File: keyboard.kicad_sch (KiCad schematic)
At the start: 101 parts, among them SW1 SW_PUSH, SW10 SW_PUSH, SW11 SW_PUSH, SW12 SW_PUSH, SW13 SW_PUSH, SW14 SW_PUSH, SW15 SW_PUSH, SW16 SW_PUSH, SW17 SW_PUSH, SW18 SW_PUSH, SW19 SW_PUSH, SW2 SW_PUSH, SW20 SW_PUSH, SW21 SW_PUSH, SW22 SW_PUSH, SW23 SW_PUSH, SW24 SW_PUSH, SW25 SW_PUSH, SW26 SW_PUSH, SW27 SW_PUSH, SW28 SW_PUSH, SW29 SW_PUSH, SW3 SW_PUSH, SW30 SW_PUSH, SW31 SW_PUSH, SW32 SW_PUSH, SW33 SW_PUSH, SW34 SW_PUSH, SW35 SW_PUSH, SW36 SW_PUSH, SW37 SW_PUSH, SW38 SW_PUSH, SW39 SW_PUSH, SW4 SW_PUSH, SW40 SW_PUSH, SW41 SW_PUSH, SW42 SW_PUSH, SW43 SW_PUSH, SW5 SW_PUSH, SW6 SW_PUSH, SW7 SW_PUSH, SW8 SW_PUSH, SW9 SW_PUSH, U1 Pico

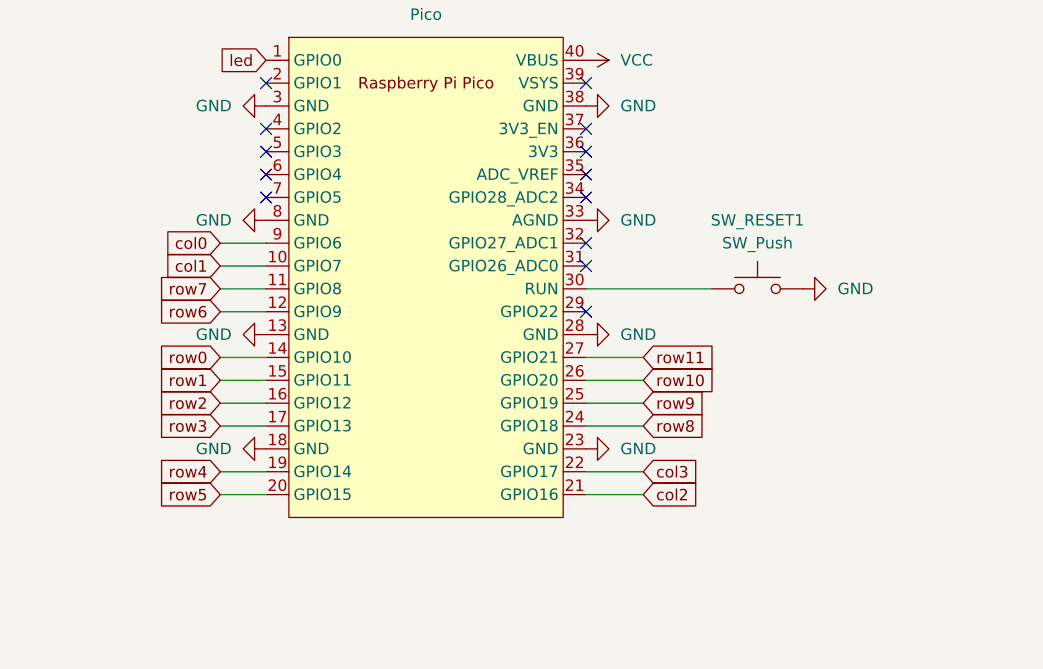
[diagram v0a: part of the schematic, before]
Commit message: :construction:
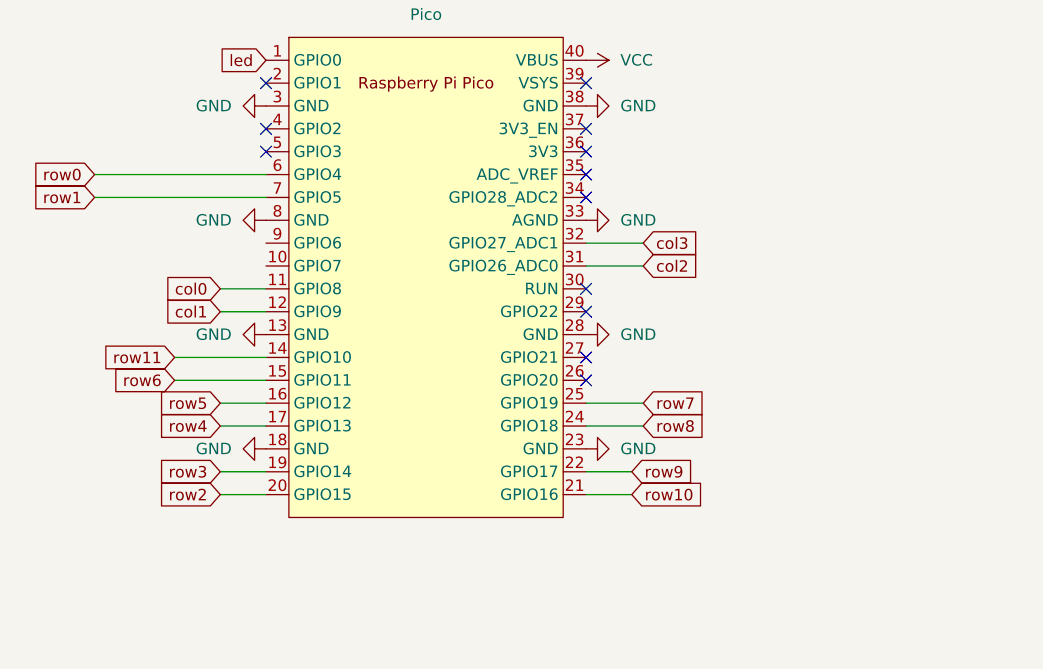
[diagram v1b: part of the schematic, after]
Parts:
- removed SW_RESET1: SW_Push, mikamo3:TactSwitch, symbol Switch:SW_Push
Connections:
- net col0: now also U1.11 (GPIO8); no longer U1.9 (GPIO6)
- net col1: now also U1.12 (GPIO9); no longer U1.10 (GPIO7)
- net col2: now also U1.31 (GPIO26_ADC0); no longer U1.21 (GPIO16)
- net col3: now also U1.32 (GPIO27_ADC1); no longer U1.22 (GPIO17)
- net row0: now also U1.6 (GPIO4); no longer U1.14 (GPIO10)
- net row1: now also U1.7 (GPIO5); no longer U1.15 (GPIO11)
- net row10: now also U1.21 (GPIO16); no longer U1.26 (GPIO20)
- net row11: now also U1.14 (GPIO10); no longer U1.27 (GPIO21)
- net row2: now also U1.20 (GPIO15); no longer U1.16 (GPIO12)
- net row3: now also U1.19 (GPIO14); no longer U1.17 (GPIO13)
- net row4: now also U1.17 (GPIO13); no longer U1.19 (GPIO14)
- net row5: now also U1.16 (GPIO12); no longer U1.20 (GPIO15)
- net row6: now also U1.15 (GPIO11); no longer U1.12 (GPIO9)
- net row7: now also U1.25 (GPIO19); no longer U1.11 (GPIO8)
- net row9: now also U1.22 (GPIO17); no longer U1.25 (GPIO19)
- no-connect marks 14 -> 13

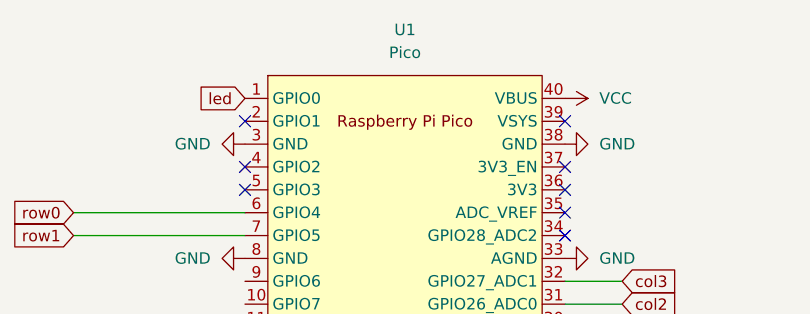
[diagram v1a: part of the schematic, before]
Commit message: :sparkles: (all) before pcb order
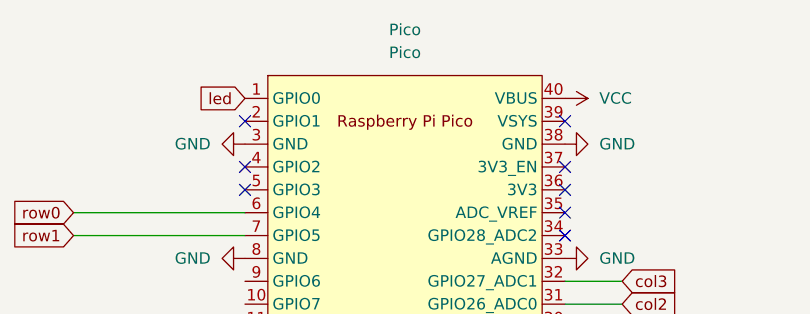
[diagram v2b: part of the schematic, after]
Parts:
- renumbered U1 to Pico
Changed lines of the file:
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@@
   (symbol (lib_id "mikamo3:Raspberry_Pi_Pico(without_debugPin)") (at 43.18 49.53 0) (unit 1)
     (in_bom yes) (on_board yes) (fields_autoplaced)
-    (property "Reference" "U1" (id 0) (at 43.18 17.78 0))
+    (property "Reference" "Pico" (id 0) (at 43.18 17.78 0))
     (property "Value" "Pico" (id 1) (at 43.18 20.32 0))
     (property "Footprint" "mikamo3:raspberry_pi_pico" (id 2) (at 43.18 49.53 90)
@@
       (reference "LED13") (unit 1) (value "YS-SK6812MINI-E") (footprint "mikamo3:YS-SK6812MINI-E")
     )
+    (path "/d62990f7-f6d3-4d28-a6c5-3edf4b260501"
+      (reference "Pico") (unit 1) (value "Pico") (footprint "mikamo3:raspberry_pi_pico")
+    )
     (path "/a4f1aa9d-559e-4977-b38d-408ec59e07b2"
       (reference "SW1") (unit 1) (value "SW_PUSH") (footprint "mikamo3:CherryMX_Hotswap_1u")
@@
       (reference "SW43") (unit 1) (value "SW_PUSH") (footprint "mikamo3:CherryMX_Hotswap_1.25u")
     )
-    (path "/d62990f7-f6d3-4d28-a6c5-3edf4b260501"
-      (reference "U1") (unit 1) (value "Pico") (footprint "mikamo3:raspberry_pi_pico")
-    )
-  )
+  )
